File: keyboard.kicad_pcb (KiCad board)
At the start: 2 copper layers, 80 x 95 mm, 75 parts, among them J1 USB_C_Receptacle_USB2.0_16P, J3 Conn_01x10_Pin, Q1 NMOS, SW1 SW_Push, SW10 SW_Push, SW11 RotaryEncoder_Switch, SW2 SW_Push, SW3 SW_Push, SW4 SW_Push, SW5 SW_Push, SW6 SW_Push, SW7 SW_Push, SW8 SW_Push, SW9 SW_Push, U1 STM32F072CBT6, U2 USBLC6-2P6, U3 SN74LV1T34DBV, U4 LDO40LPU33RY, U5 SN74LV1T34DBV

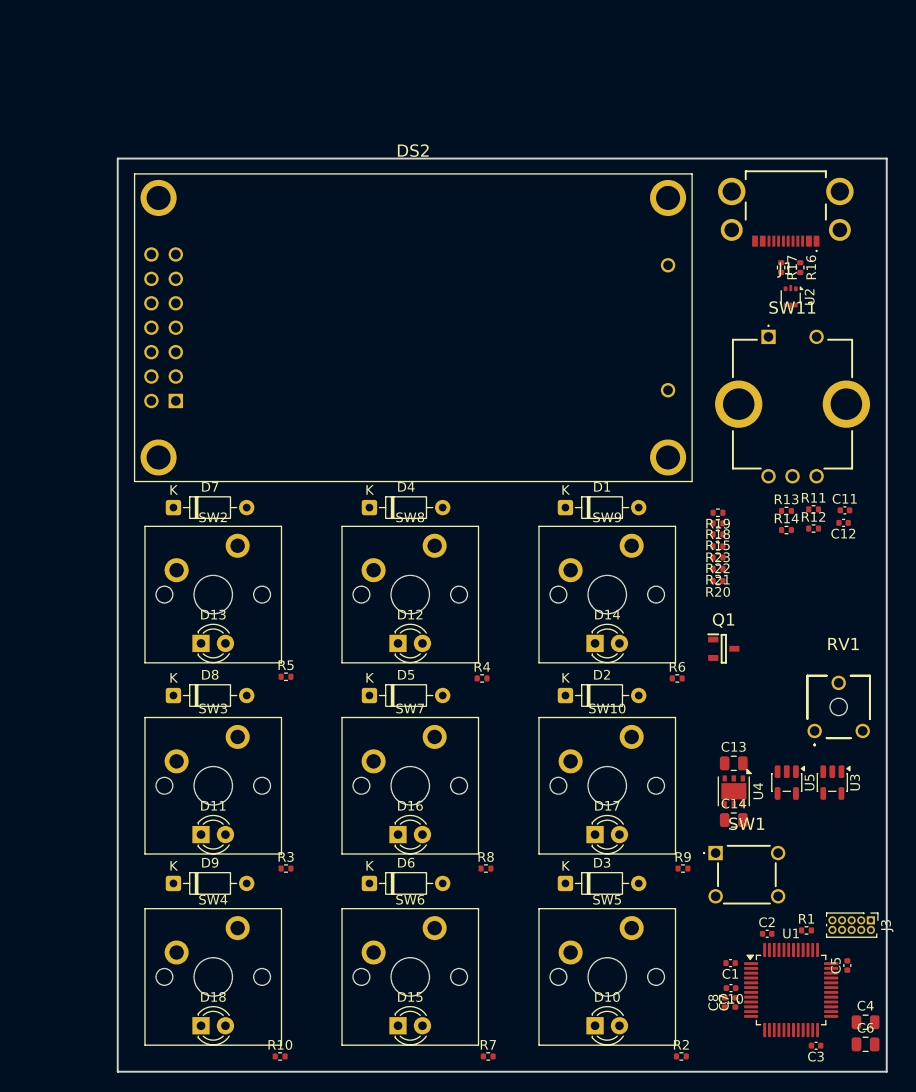
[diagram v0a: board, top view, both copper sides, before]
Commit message: Added pcb routing
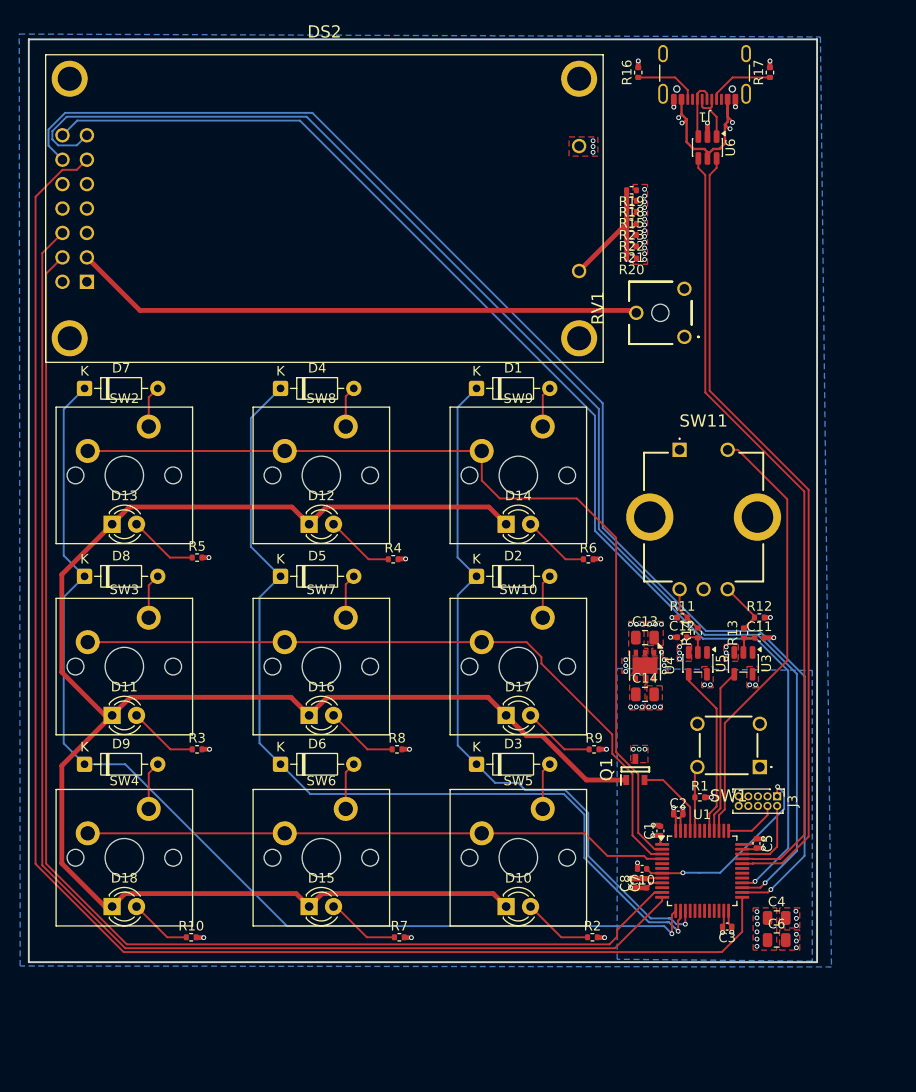
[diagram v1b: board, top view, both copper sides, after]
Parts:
- removed U2: USBLC6-2P6, Package_TO_SOT_SMD:SOT-666
- added U6: USBLC6-2SC6, Package_TO_SOT_SMD:SOT-23-6, F.Cu at (189.4, 54.8)
- J1: footprint my_footprints:UJ20CHGMSMT4BP16TR -> Connector_USB:USB_C_Receptacle_GCT_USB4105-xx-A_16P_TopMnt_Horizontal
- moved RV1 43.2 mm to (187.0, 74.5), turned to 90 degrees
- moved R20 34.7 mm to (181.5, 66.3)
- moved R18 34.7 mm to (181.5, 60.4)
- moved R22 34.7 mm to (181.5, 63.9)
- moved R15 34.7 mm to (181.5, 61.5)
- moved R19 34.7 mm to (181.5, 59.2)
- moved R21 34.7 mm to (181.5, 65.1)
- moved R23 34.7 mm to (181.5, 62.8)
- moved R16 26.4 mm to (182.2, 47.0), turned to 90 degrees
- moved C12 20.6 mm to (186.8, 105.8), turned to 0 degrees
- moved R17 20.3 mm to (195.9, 47.0), turned to 90 degrees
- moved R1 17.7 mm to (188.6, 122.4)
- moved R11 17.7 mm to (186.8, 103.7)
- moved J1 17.0 mm to (189.1, 46.1)
- moved J3 16.2 mm to (196.7, 122.3)
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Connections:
- C14 pad 1: +3V3 -> +3.3V
- J3 pad 2: /SWCLK -> /SWDIO
- J3 pad 4: /SWDIO -> /SWCLK
- U1 pad 11: unconnected-(U1-PA1-Pad11) -> /LCD_RS
- U1 pad 12: unconnected-(U1-PA2-Pad12) -> /LCD_ENABLE
- U1 pad 13: unconnected-(U1-PA3-Pad13) -> Row 1
- U1 pad 14: unconnected-(U1-PA4-Pad14) -> Row 2
- U1 pad 15: Column 3 -> Row 3
- U1 pad 16: Column 2 -> unconnected-(U1-PA6-Pad16)
- U1 pad 17: Column 1 -> unconnected-(U1-PA7-Pad17)
- U1 pad 2: unconnected-(U1-PC13-Pad2) -> Column 1
- U1 pad 21: /LCD_ENABLE -> unconnected-(U1-PB10-Pad21)
- U1 pad 22: /DB4 -> unconnected-(U1-PB11-Pad22)
- U1 pad 25: /DB5 -> /DB4
- U1 pad 26: /DB6 -> /DB5
- U1 pad 27: /DB7 -> /DB6
- U1 pad 28: unconnected-(U1-PB15-Pad28) -> /DB7
- U1 pad 29: Row 3 -> unconnected-(U1-PA8-Pad29)
- U1 pad 3: unconnected-(U1-PC14-Pad3) -> Column 2
- U1 pad 30: Row 2 -> unconnected-(U1-PA9-Pad30)
- U1 pad 31: Row 1 -> unconnected-(U1-PA10-Pad31)
- U1 pad 39: unconnected-(U1-PB3-Pad39) -> /MUTE
- U1 pad 4: unconnected-(U1-PC15-Pad4) -> Column 3
- U1 pad 40: /OUT_A -> /OUT_B
- U1 pad 41: /OUT_B -> /OUT_A
- U1 pad 43: /MUTE -> unconnected-(U1-PB7-Pad43)
- U1 pad 46: /LCD_RS -> unconnected-(U1-PB9-Pad46)
- U3 pad 5: +3V3 -> +3.3V
- U4 pad 4: +3V3 -> +3.3V
- U4 pad 5: +3V3 -> +3.3V
- U5 pad 5: +3V3 -> +3.3V
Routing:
- net Net-(D10-K): track 0.00 -> 195.9 mm
- net /DB4: track 0.00 -> 158.2 mm
- net /DB5: track 0.00 -> 141.7 mm, vias 0 -> 1
- net /DB6: track 0.00 -> 140.3 mm, vias 0 -> 1
- net /LCD_ENABLE: track 0.00 -> 137.1 mm
- net /LCD_RS: track 0.00 -> 134.0 mm
- net /DB7: track 0.00 -> 131.6 mm, vias 0 -> 1
- net Row 1: track 0.00 -> 113.7 mm, vias 0 -> 1
- net Row 2: track 0.00 -> 96.9 mm, vias 0 -> 1
- net Column 1: track 0.00 -> 95.4 mm
- net /USB_D-: track 0.00 -> 83.2 mm
- net /USB_D+: track 0.00 -> 82.5 mm
- net Row 3: track 0.00 -> 75.0 mm, vias 0 -> 1
- net Column 2: track 0.00 -> 74.2 mm
- net Column 3: track 0.00 -> 60.9 mm
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- added copper zone on B.Cu, net +3.3V
- added copper zone on F.Cu, net +3.3V
- added copper zone on B.Cu, net +5V
- added copper zone on F.Cu, net +5V
- added copper zone on F.Cu, net GND
- added copper zone on In1.Cu, net GND
- added copper zone on In2.Cu, net GND
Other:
- board size 80 x 95 mm -> 82 x 96 mm
- copper layers 2 -> 4
